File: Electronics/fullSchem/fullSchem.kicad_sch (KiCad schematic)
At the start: 1 part, among them U1 Teensy4.1

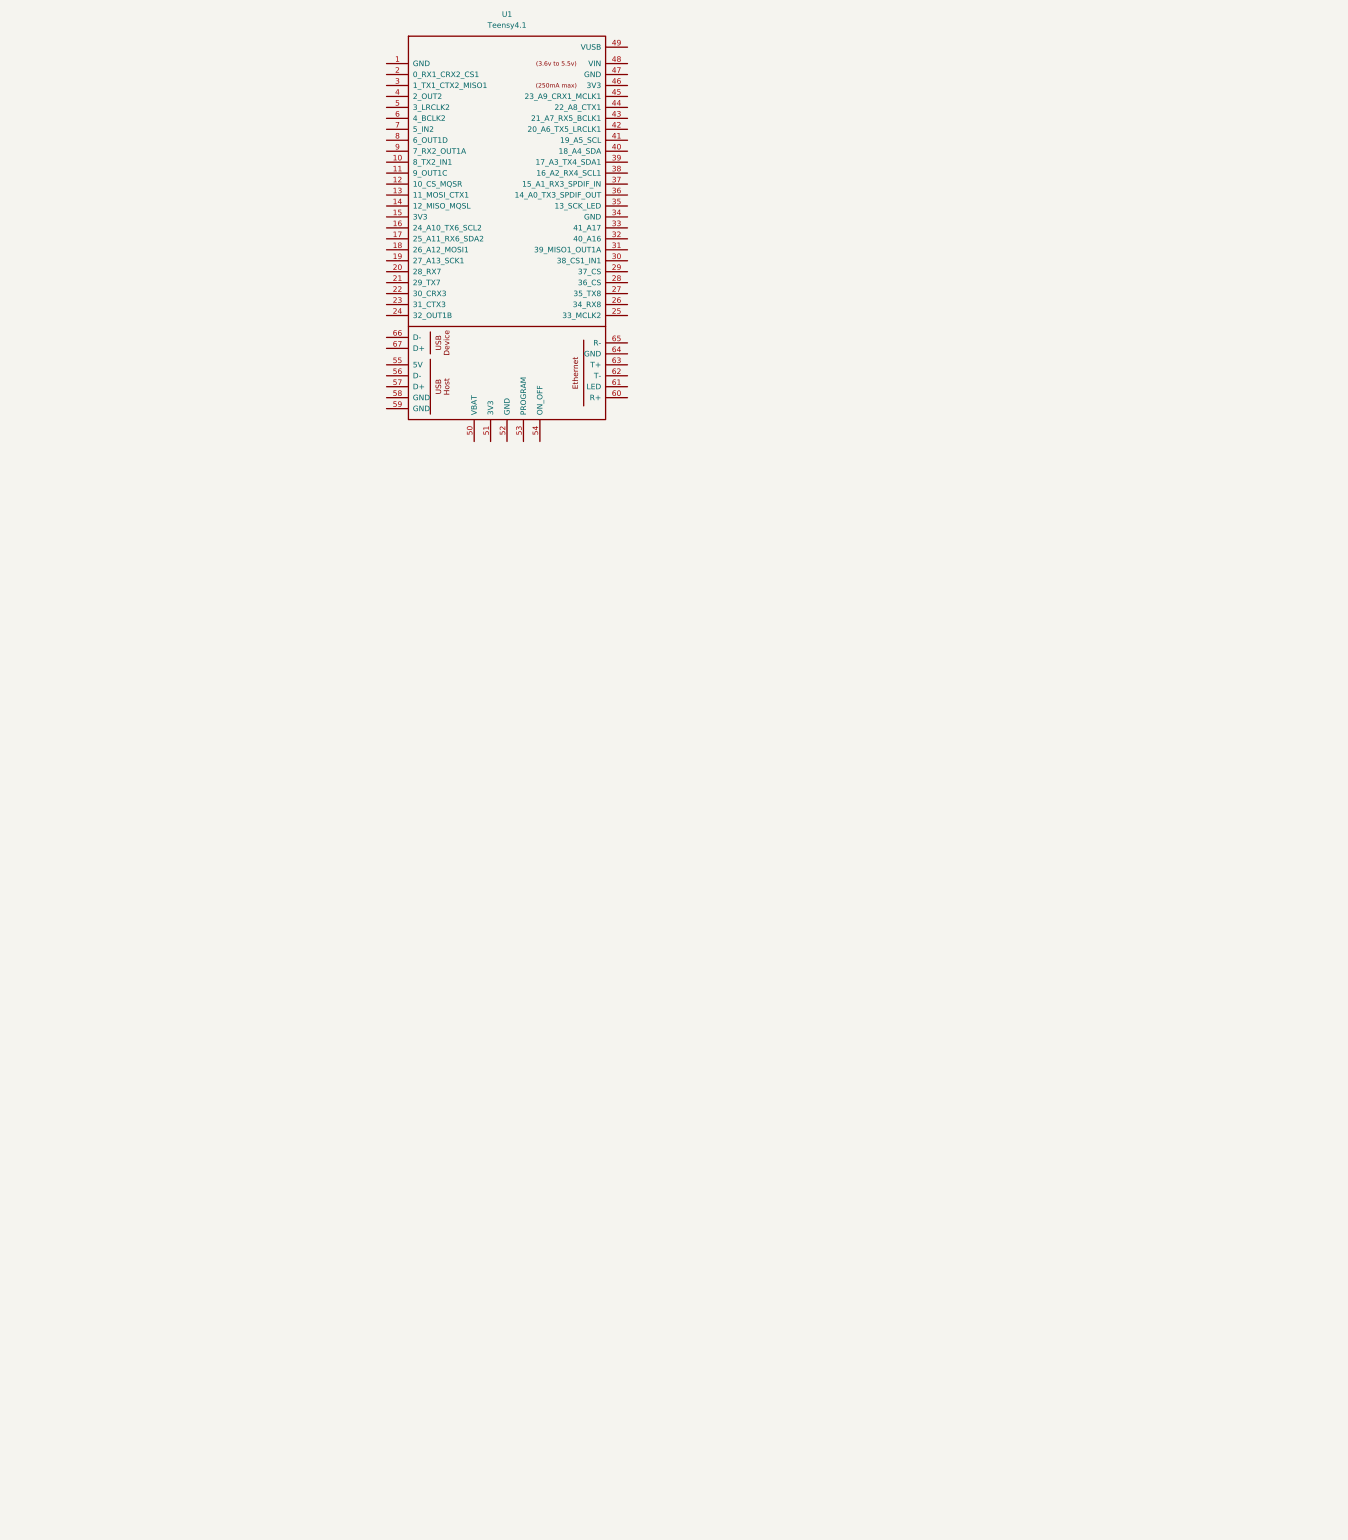
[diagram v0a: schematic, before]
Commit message: scaffolding for fullSchem
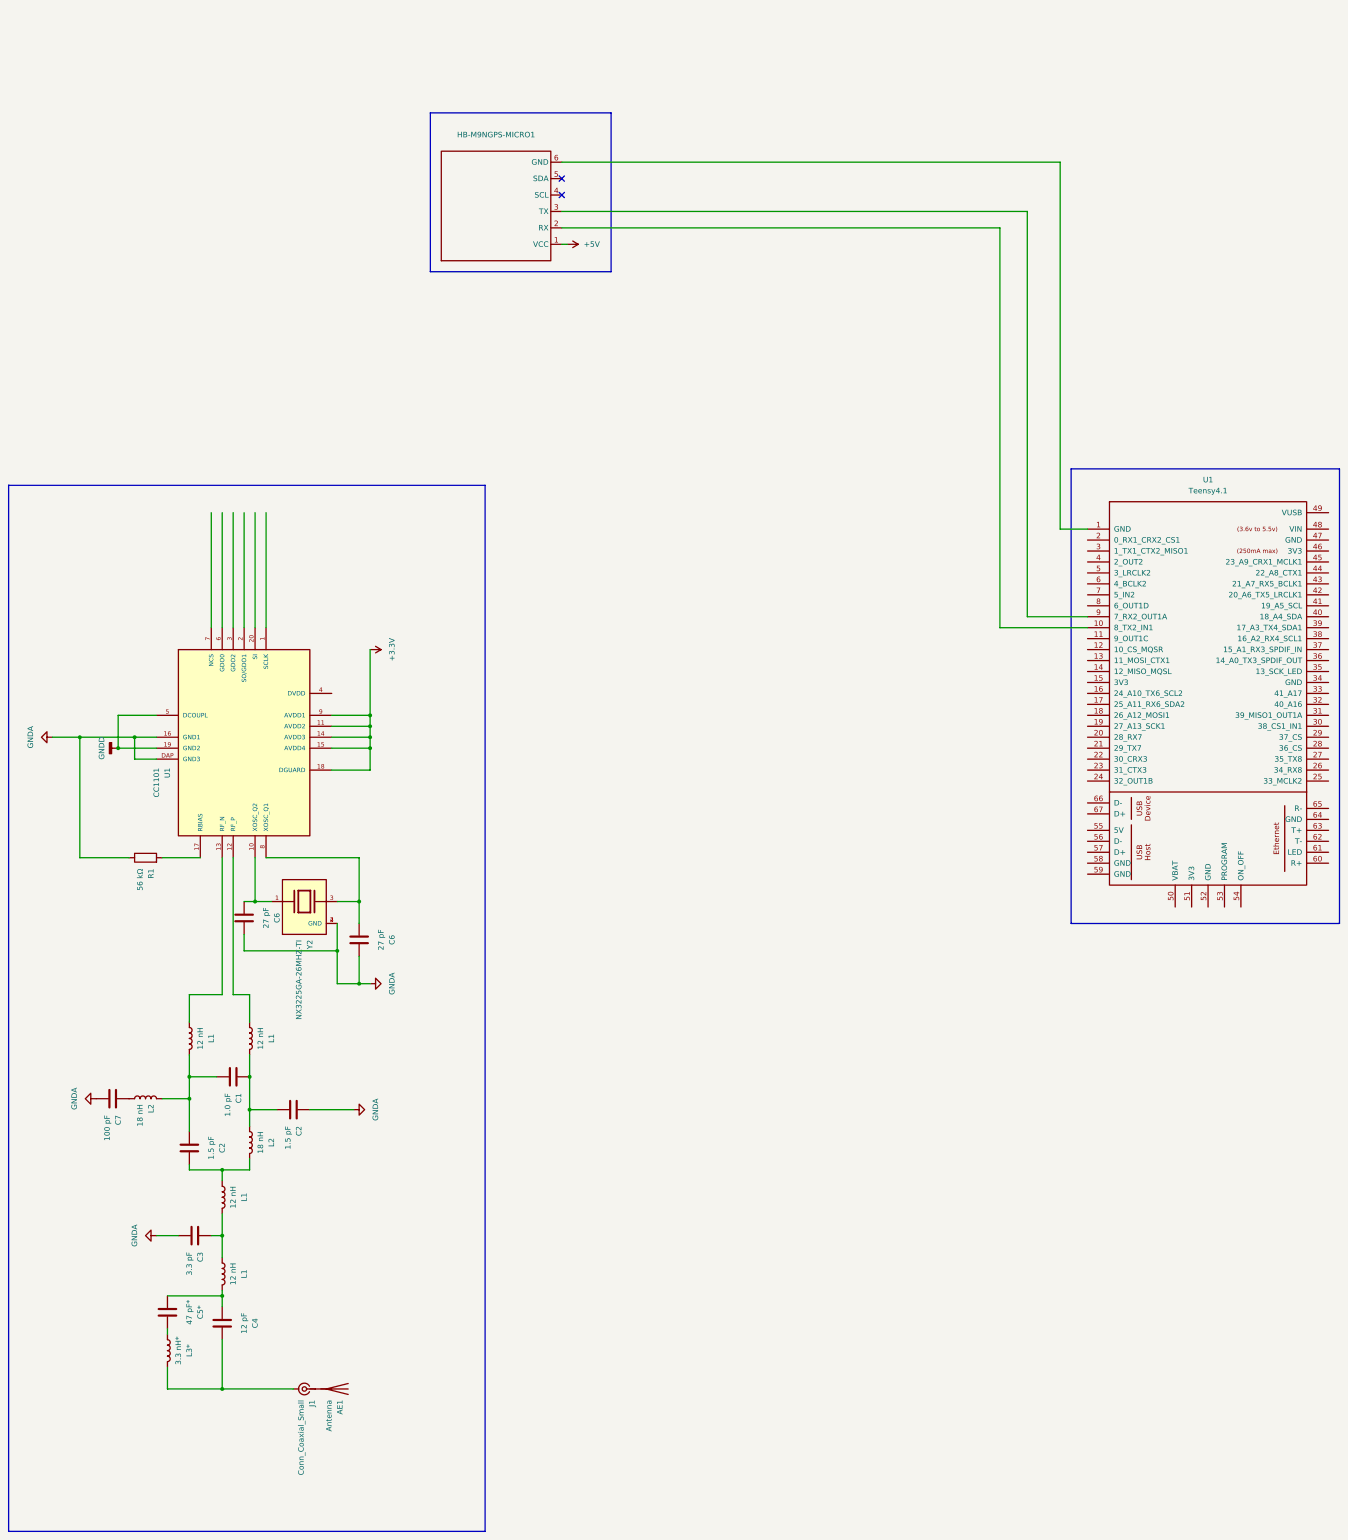
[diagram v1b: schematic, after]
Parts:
- added AE1: Antenna, symbol Device:Antenna
- added C1: 1.0 pF, symbol Device:C
- added C2 (x2): 1.5 pF, symbol Device:C
- added C3: 3.3 pF, symbol Device:C
- added C4: 12 pF, symbol Device:C
- added C5*: 47 pF*, symbol Device:C
- added C6 (x2): 27 pF, symbol Device:C
- added C7: 100 pF, symbol Device:C
- added HB-M9NGPS-MICRO1: ~, symbol addlSymbols:HolybroMicroM9N
- added J1: Conn_Coaxial_Small, symbol Connector:Conn_Coaxial_Small
- added L1 (x4): 12 nH, symbol Device:L
- added L2 (x2): 18 nH, symbol Device:L
- added L3*: 3.3 nH*, symbol Device:L
- added R1: 56 kΩ, symbol Device:R
- added U1: CC1101, CC1101:QLP20, symbol CC1101:CC1101
- added Y2: NX3225GA-26MHZ-TI, NX3225GA-26MHZ-TI:OSCCC320X250X90N, symbol NX3225GA-26MHZ-TI:NX3225GA-26MHZ-TI
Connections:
- net at U1.1 (GND): now also HB-M9NGPS-MICRO1.6 (GND)
- net at U1.10 (8_TX2_IN1): now also HB-M9NGPS-MICRO1.2 (RX)
- net at U1.9 (7_RX2_OUT1A): now also HB-M9NGPS-MICRO1.3 (TX)
- new net: C2.1, L1.1, L2.2
- new net: C3.1, L1.1, L1.2
- new net: C1.1, C2.2, L1.2, L2.1
- new net: AE1.1 (A), J1.1 (In)
- new net: C4.2, J1.2 (Ext), L3*.2
- new net: C4.1, C5*.1, L1.2
- new net: C5*.2, L3*.1
- new net: C1.2, C2.2, L1.2, L2.2
- new net: R1.2, U1.17 (RBIAS)
- new net: C6.2, U1.10 (XOSC_Q2), Y2.1
- new net: C6.1, U1.8 (XOSC_Q1), Y2.3
- new net: L1.1, U1.12 (RF_P)
- new net: C7.2, L2.1
- new net: L1.1, U1.13 (RF_N)
- new net +3.3V: U1.11 (AVDD2), U1.14 (AVDD3), U1.15 (AVDD4), U1.18 (DGUARD), U1.9 (AVDD1)
- new net +5V: HB-M9NGPS-MICRO1.1 (VCC)
- new net GNDA: C2.1, C3.2, C6.1, C6.2, C7.1, R1.1, U1.16 (GND1), U1.DAP (GND3), Y2.2 (GND), Y2.4 (GND)
- new net GNDD: U1.19 (GND2), U1.5 (DCOUPL)
- no-connect marks 0 -> 2
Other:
- moved on the sheet: U1
